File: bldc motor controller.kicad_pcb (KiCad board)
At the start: 4 copper layers, 26 x 26 mm, 58 parts, among them J1 Conn_01x04_Pin, M2 MountingHole_2.2mm_M2_DIN965_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, U1 C47023655, U2 ISM330DHCXTR, U3 C529358, U6 LIS2MDLTR

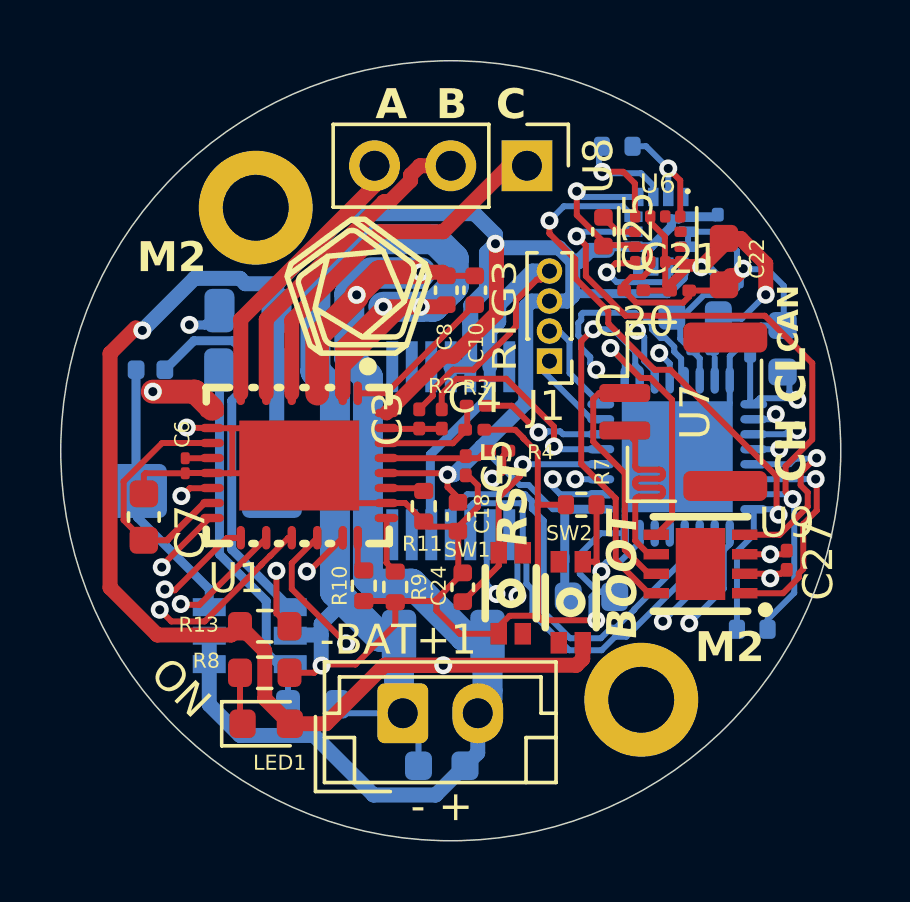
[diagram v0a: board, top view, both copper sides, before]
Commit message: 3.3v plane, finale besides that
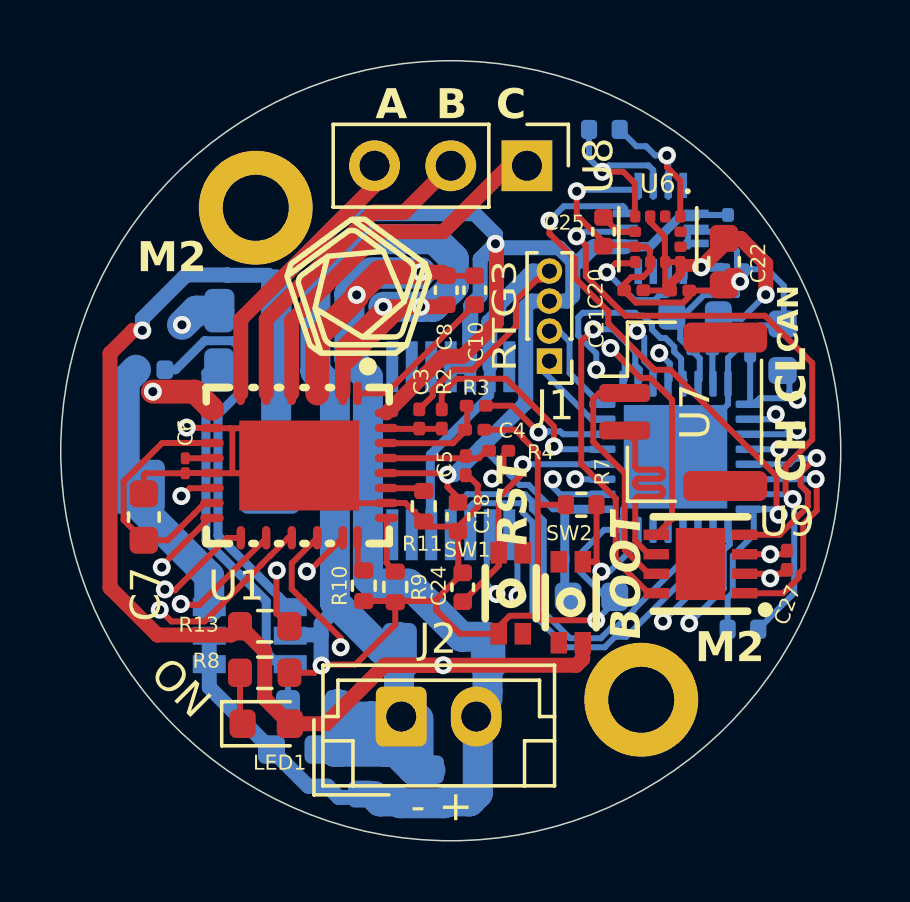
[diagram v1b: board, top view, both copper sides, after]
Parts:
- removed -BAT+1: ~, Connector_JST:JST_EH_B2B-EH-A_1x02_P2.50mm_Vertical
- removed U3: C529358, bldc-motor-footprints:QFN-32_L5.0-W5.0-P0.50-BL-EP3.7
- added C28: 10 uf, Capacitor_SMD:C_0603_1608Metric, B.Cu at (137.3, 98.0)
- added C29: 10 uf, Capacitor_SMD:C_0603_1608Metric, B.Cu at (139.4, 92.5)
- added C30: 10 uf, Capacitor_SMD:C_0603_1608Metric, B.Cu at (139.6, 98.7)
- added J2: Conn_01x02, Connector_JST:JST_EH_B2B-EH-A_1x02_P2.50mm_Vertical, F.Cu at (140.8, 96.9)
- added U10: STM32G431KBUx, Package_DFN_QFN:QFN-32-1EP_5x5mm_P0.5mm_EP3.45x3.45mm, B.Cu at (150.0, 88.2)
- U2: value ISM330DHCXTR -> LSM6DSV16XTR; footprint bldc-motor-footprints:PQFN50P250X300X86-14N -> bldc-motor-footprints:LGA-14L_STM
- moved R12 0.71 mm to (147.6, 77.3)
- moved C23 0.48 mm to (151.9, 82.0)
- moved C1 0.44 mm to (142.3, 94.6)
- moved C9 0.42 mm to (142.6, 98.6)
- moved C26 0.34 mm to (151.7, 80.5)
- moved R5 0.31 mm to (152.2, 94.0)
- moved L1 0.16 mm to (134.2, 89.2)
- moved U2 0.11 mm to (149.5, 80.6)
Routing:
- net -BATT: track 40.9 -> 52.4 mm
- net GND: track 97.6 -> 102.2 mm
- net TIM1_CH3N: track 22.6 -> 18.5 mm
- net +3.3V: track 188.4 -> 186.8 mm
- net TI_AVDD: track 10.0 -> 8.51 mm
- net PHASE-B: track 10.3 -> 11.6 mm
- net MSDA: track 5.46 -> 6.80 mm
- net MSCL: track 4.31 -> 5.55 mm
- net +BATT: track 53.9 -> 54.4 mm
- net MDRDY: track 3.65 -> 4.17 mm
- added copper zone on In2.Cu, net +3.3V
- removed copper zone on In1.Cu, net (none)
